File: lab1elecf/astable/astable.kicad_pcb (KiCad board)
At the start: 2 copper layers, 50 x 50 mm, 7 parts, among them J1 Conn_01x02, J2 Conn_01x02, U1 ICM7555xB

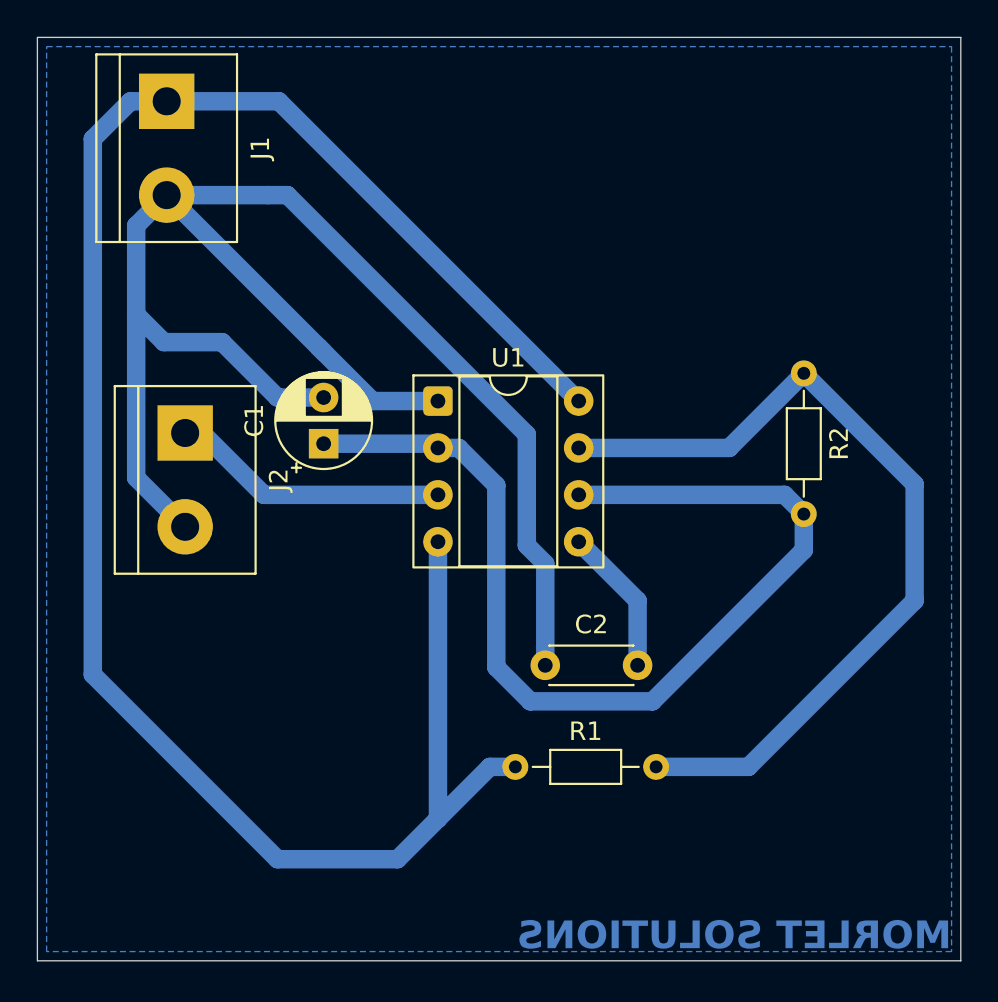
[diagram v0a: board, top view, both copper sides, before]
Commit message: VCC Y GND
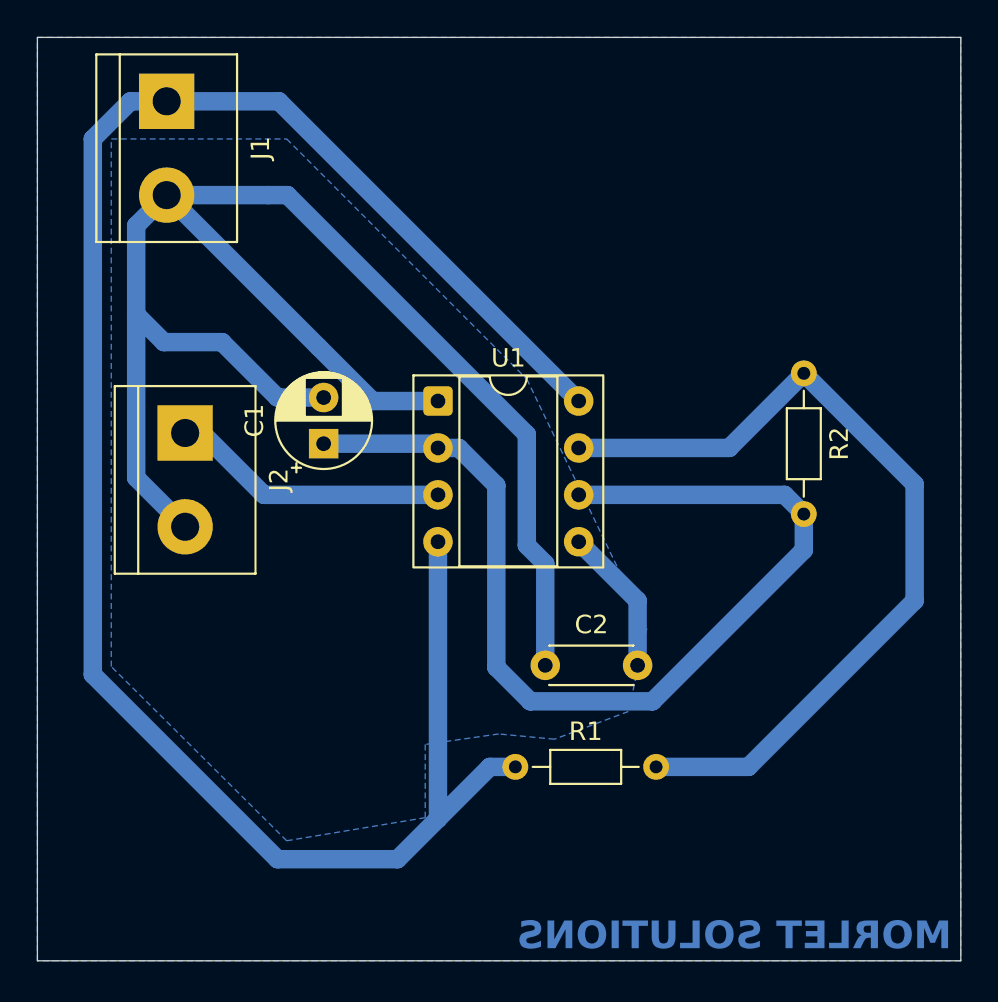
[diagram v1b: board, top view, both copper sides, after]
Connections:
- net Net-(J1-Pin_1) renamed VCC
- net Net-(J1-Pin_2) renamed GND
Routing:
- added copper zone on B.Cu, net GND
- added copper zone on B.Cu, net VCC
- removed copper zone on B.Cu, net (none)
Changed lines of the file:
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@@
 	)
 	(net 0 "")
-	(net 1 "Net-(J1-Pin_2)")
+	(net 1 "GND")
 	(net 2 "Net-(U1-THR)")
 	(net 3 "Net-(U1-CV)")
-	(net 4 "Net-(J1-Pin_1)")
+	(net 4 "VCC")
 	(net 5 "Net-(J2-Pin_1)")
 	(net 6 "Net-(U1-DIS)")
@@
 		(property ki_fp_filters "C_*")
 		(sheetname "/")
-		(sheetfile "monomono.kicad_sch")
+		(sheetfile "astable.kicad_sch")
 		(attr through_hole)
 		(fp_line
@@
 			(layers "*.Cu" "*.Mask")
 			(remove_unused_layers no)
-			(net 1 "Net-(J1-Pin_2)")
+			(net 1 "GND")
 			(pintype "passive")
 		)
@@
 		(property ki_fp_filters "Connector*:*_1x??_*")
 		(sheetname "/")
-		(sheetfile "monomono.kicad_sch")
+		(sheetfile "astable.kicad_sch")
 		(attr through_hole)
 		(fp_line
@@
 			(layers "*.Cu" "*.Mask")
 			(remove_unused_layers no)
-			(net 1 "Net-(J1-Pin_2)")
+			(net 1 "GND")
 			(pinfunction "Pin_2")
 			(pintype "passive")
@@
 		(property ki_fp_filters "CP_*")
 		(sheetname "/")
-		(sheetfile "monomono.kicad_sch")
+		(sheetfile "astable.kicad_sch")
 		(attr through_hole)
 		(fp_line
@@
 			(layers "*.Cu" "*.Mask")
 			(remove_unused_layers no)
-			(net 1 "Net-(J1-Pin_2)")
+			(net 1 "GND")
 			(pintype "passive")
 		)
@@
 		(property ki_fp_filters "R_*")
 		(sheetname "/")
-		(sheetfile "monomono.kicad_sch")
+		(sheetfile "astable.kicad_sch")
 		(attr through_hole)
 		(fp_line
@@
 		(property ki_fp_filters "SOIC*3.9x4.9mm*P1.27mm*")
 		(sheetname "/")
-		(sheetfile "monomono.kicad_sch")
+		(sheetfile "astable.kicad_sch")
 		(attr through_hole)
 		(fp_line
@@
 			(remove_unused_layers no)
 			(roundrect_rratio 0.15625)
-			(net 1 "Net-(J1-Pin_2)")
+			(net 1 "GND")
 			(pinfunction "GND")
 			(pintype "power_in")
@@
 			(layers "*.Cu" "*.Mask")
 			(remove_unused_layers no)
-			(net 4 "Net-(J1-Pin_1)")
+			(net 4 "VCC")
 			(pinfunction "R")
 			(pintype "input")
@@
 			(layers "*.Cu" "*.Mask")
 			(remove_unused_layers no)
-			(net 4 "Net-(J1-Pin_1)")
+			(net 4 "VCC")
 			(pinfunction "VCC")
 			(pintype "power_in")
@@
 		(property ki_fp_filters "R_*")
 		(sheetname "/")
-		(sheetfile "monomono.kicad_sch")
+		(sheetfile "astable.kicad_sch")
 		(attr through_hole)
 		(fp_line
@@
 			(layers "*.Cu" "*.Mask")
 			(remove_unused_layers no)
-			(net 4 "Net-(J1-Pin_1)")
+			(net 4 "VCC")
 			(pintype "passive")
 		)
@@
 		(property ki_fp_filters "Connector*:*_1x??_*")
 		(sheetname "/")
-		(sheetfile "monomono.kicad_sch")
+		(sheetfile "astable.kicad_sch")
 		(attr through_hole)
 		(fp_line
@@
 			(layers "*.Cu" "*.Mask")
 			(remove_unused_layers no)
-			(net 4 "Net-(J1-Pin_1)")
+			(net 4 "VCC")
 			(pinfunction "Pin_1")
 			(pintype "passive")
@@
 			(layers "*.Cu" "*.Mask")
 			(remove_unused_layers no)
-			(net 1 "Net-(J1-Pin_2)")
+			(net 1 "GND")
 			(pinfunction "Pin_2")
 			(pintype "passive")
@@
 	)
 	(segment
-		(start 65.5 67.04)
-		(end 65.23 66.77)
-		(width 1)
-		(layer "B.Cu")
-		(net 1)
-	)
-	(segment
 		(start 55.349 60.191)
 		(end 57 58.54)
@@
 	)
 	(zone
-		(net 0)
-		(net_name "")
+		(net 4)
+		(net_name "VCC")
+		(layer "B.Cu")
+		(hatch edge 0.5)
+		(priority 1)
+		(connect_pads
+			(clearance 0.5)
+		)
+		(min_thickness 0.25)
+		(filled_areas_thickness no)
+		(fill yes
+			(thermal_gap 0.5)
+			(thermal_bridge_width 0.5)
+		)
+		(polygon
+			(pts
+				(xy 50 50) (xy 100 50) (xy 100 100) (xy 50 100)
+			)
+		)
+	)
+	(zone
+		(net 1)
+		(net_name "GND")
 		(layer "B.Cu")
 		(hatch edge 0.5)
@@
 			(thermal_gap 0.5)
 			(thermal_bridge_width 0.5)
-			(island_removal_mode 1)
-			(island_area_min 10)
 		)
 		(polygon
 			(pts
-				(xy 50.5 50.5) (xy 99.5 50.5) (xy 99.5 99.5) (xy 50.5 99.5)
+				(xy 54 55.5) (xy 63.5 55.5) (xy 76.5 68.5) (xy 83 82) (xy 82 86.5) (xy 78 88) (xy 74.97951 87.717221)
+				(xy 71 88.285722) (xy 71 92.25) (xy 63.5 93.5) (xy 54 84.068182)
 			)
 		)
